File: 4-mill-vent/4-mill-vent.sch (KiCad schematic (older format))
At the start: 73 parts, among them J1 Fan, J2 Buzzer, J3 Power, J4 ICSP, Q1 MMBT3904, Q2 MMBT3904, Q3 PZT3904, Q4 PZT3904, Q5 TSM480P06CP, Q6 MMBT3904, SW1 Power_off, SW2 Power_On, SW3 Fan_Down, SW4 Fan_Up, U1 LM321, U2 TPSM84212EAB, U3 LM1117-5.0, U4 ATmega328P-AU, Y1 16.000MHZ

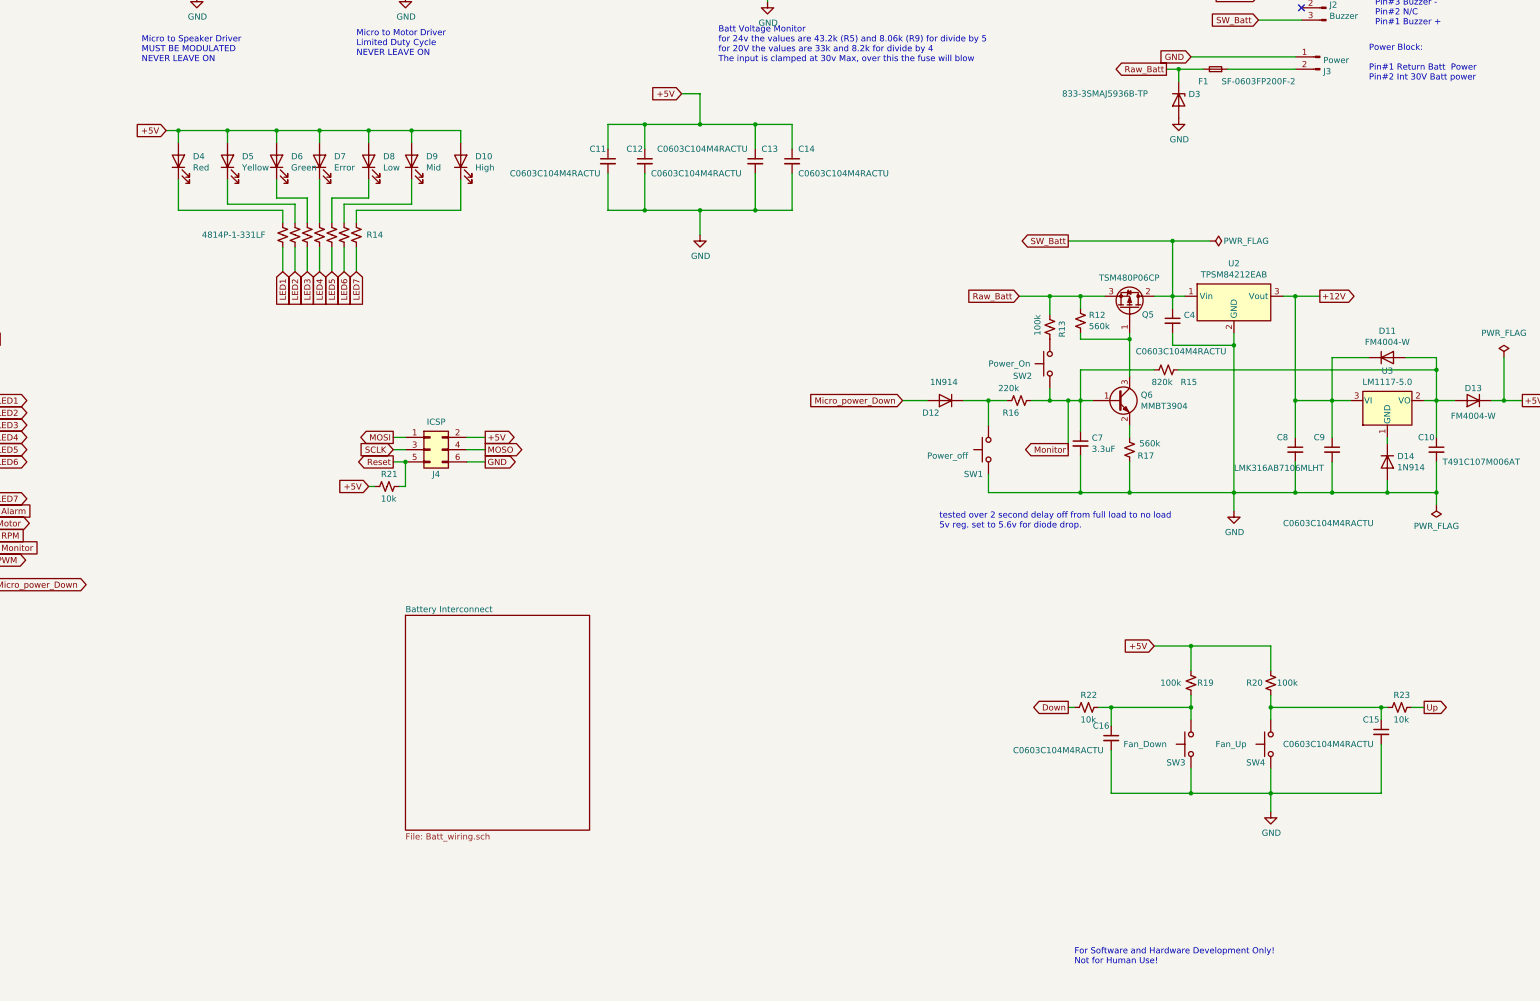
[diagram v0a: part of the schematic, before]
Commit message: lastest updates to board
Board is done, just need to do more checking
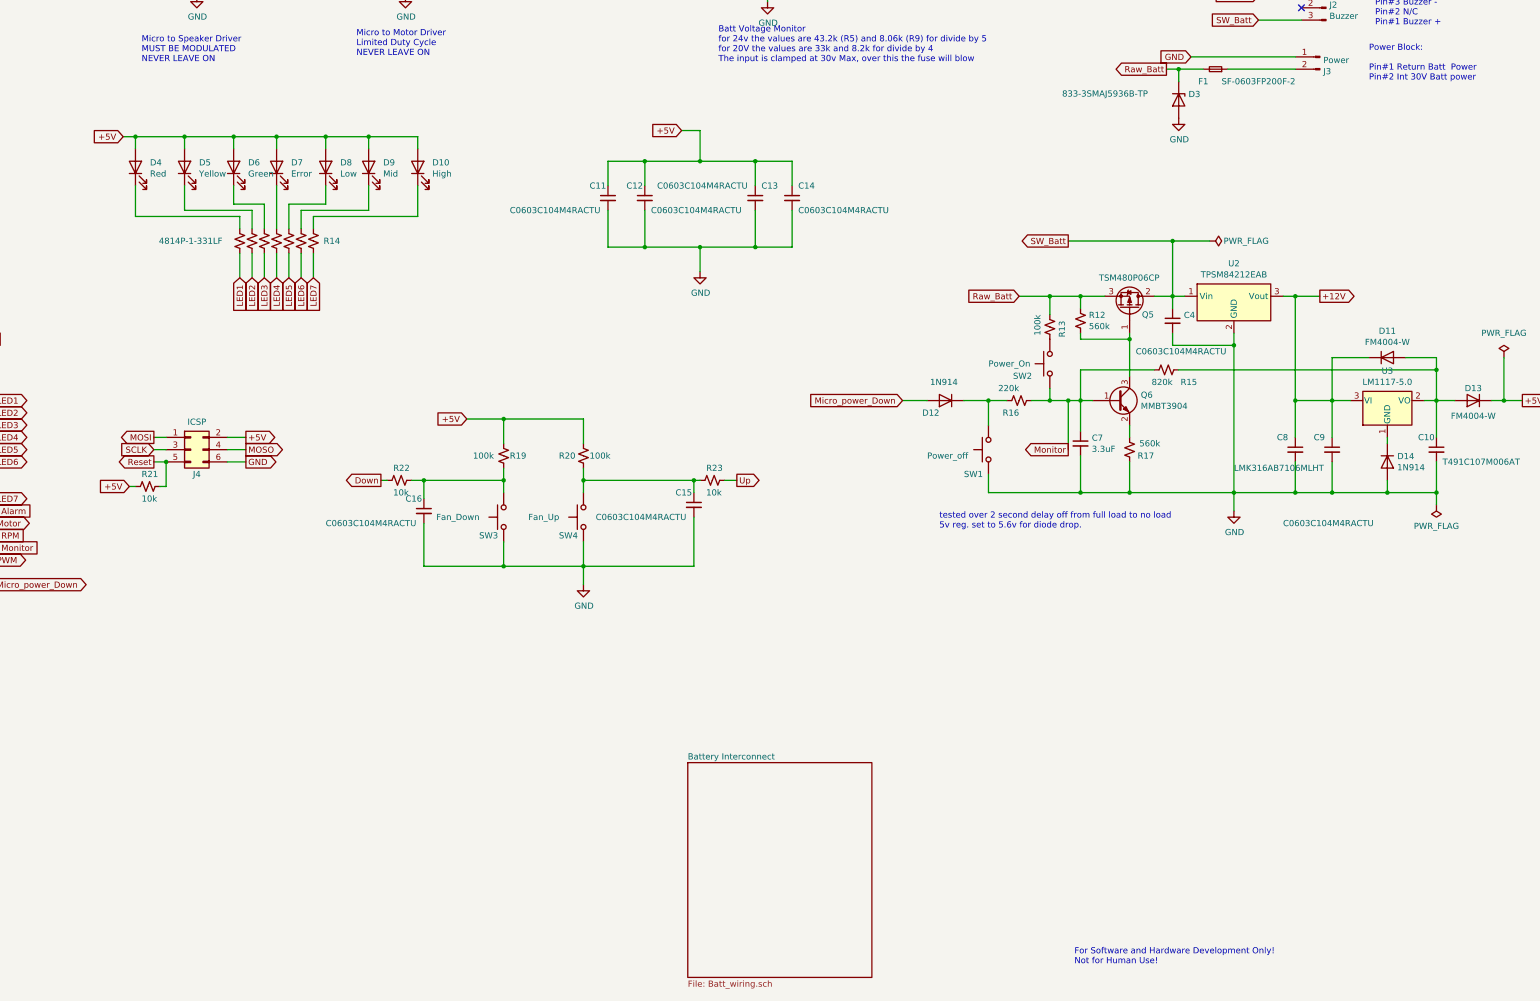
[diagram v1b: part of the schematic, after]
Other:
- moved on the sheet: C11, C12, C13, C14, C15, C16, D10, D4, D5, D6, D7, D8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
